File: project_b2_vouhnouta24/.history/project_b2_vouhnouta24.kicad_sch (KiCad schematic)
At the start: 7 parts, among them J1 AVR-ISP-10, U1 ATmega328-P-A, Y1 16Mhz

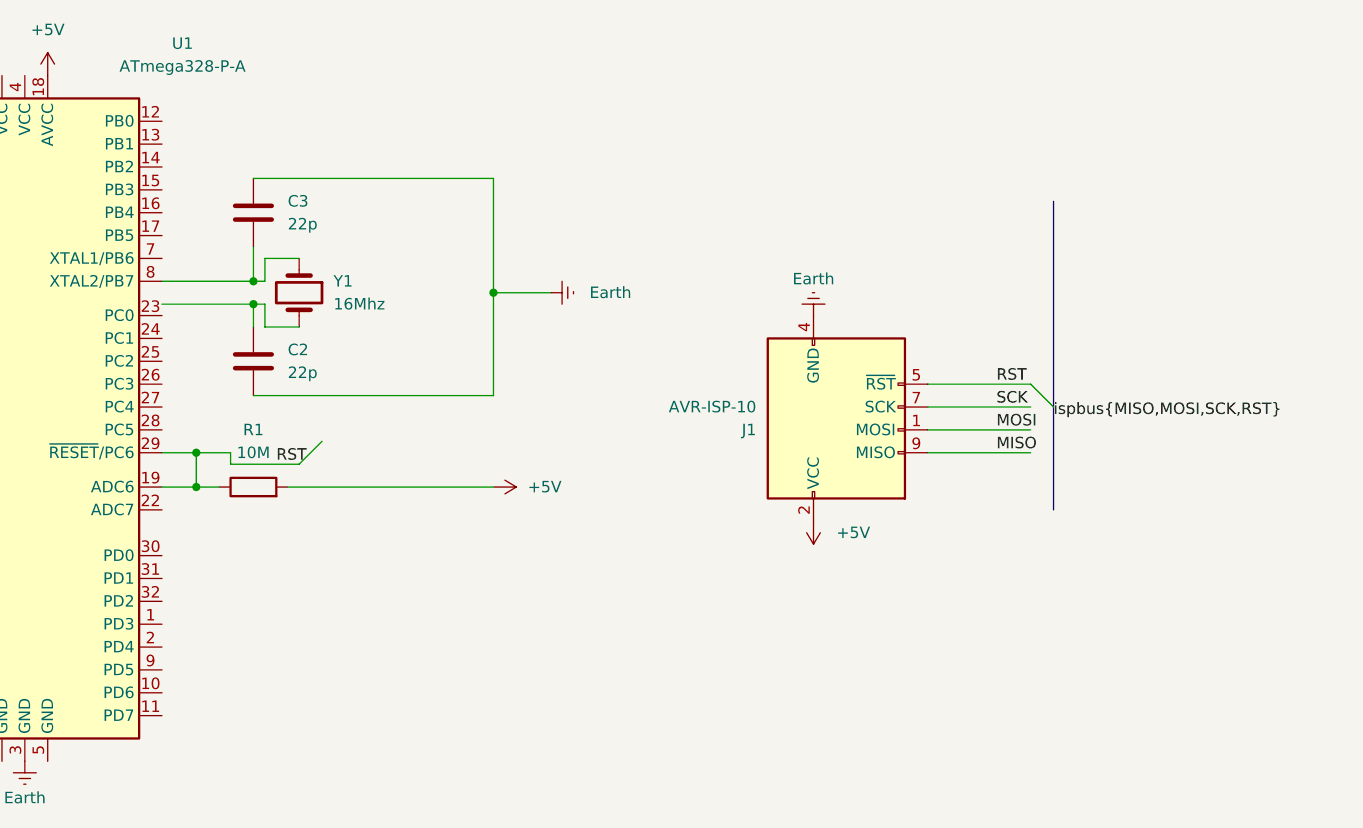
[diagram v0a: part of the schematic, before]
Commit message: J1 bus complete
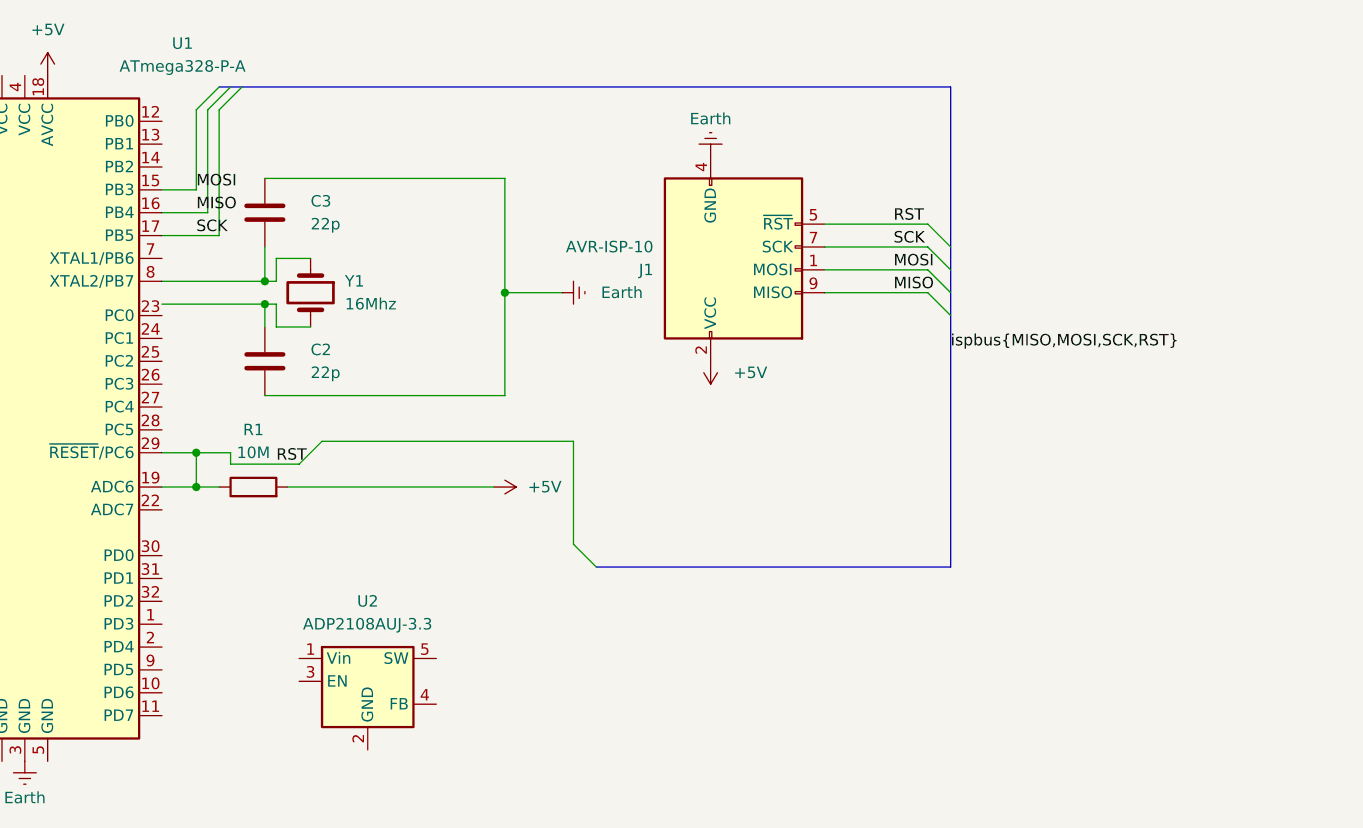
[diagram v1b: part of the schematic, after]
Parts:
- added U2: ADP2108AUJ-3.3, Package_TO_SOT_SMD:TSOT-23-5, symbol Regulator_Switching:ADP2108AUJ-3.3
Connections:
- net MISO: now also U1.16 (PB4)
- net MOSI: now also U1.15 (PB3)
- net SCK: now also U1.17 (PB5)
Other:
- moved on the sheet: C2, C3, J1, Y1

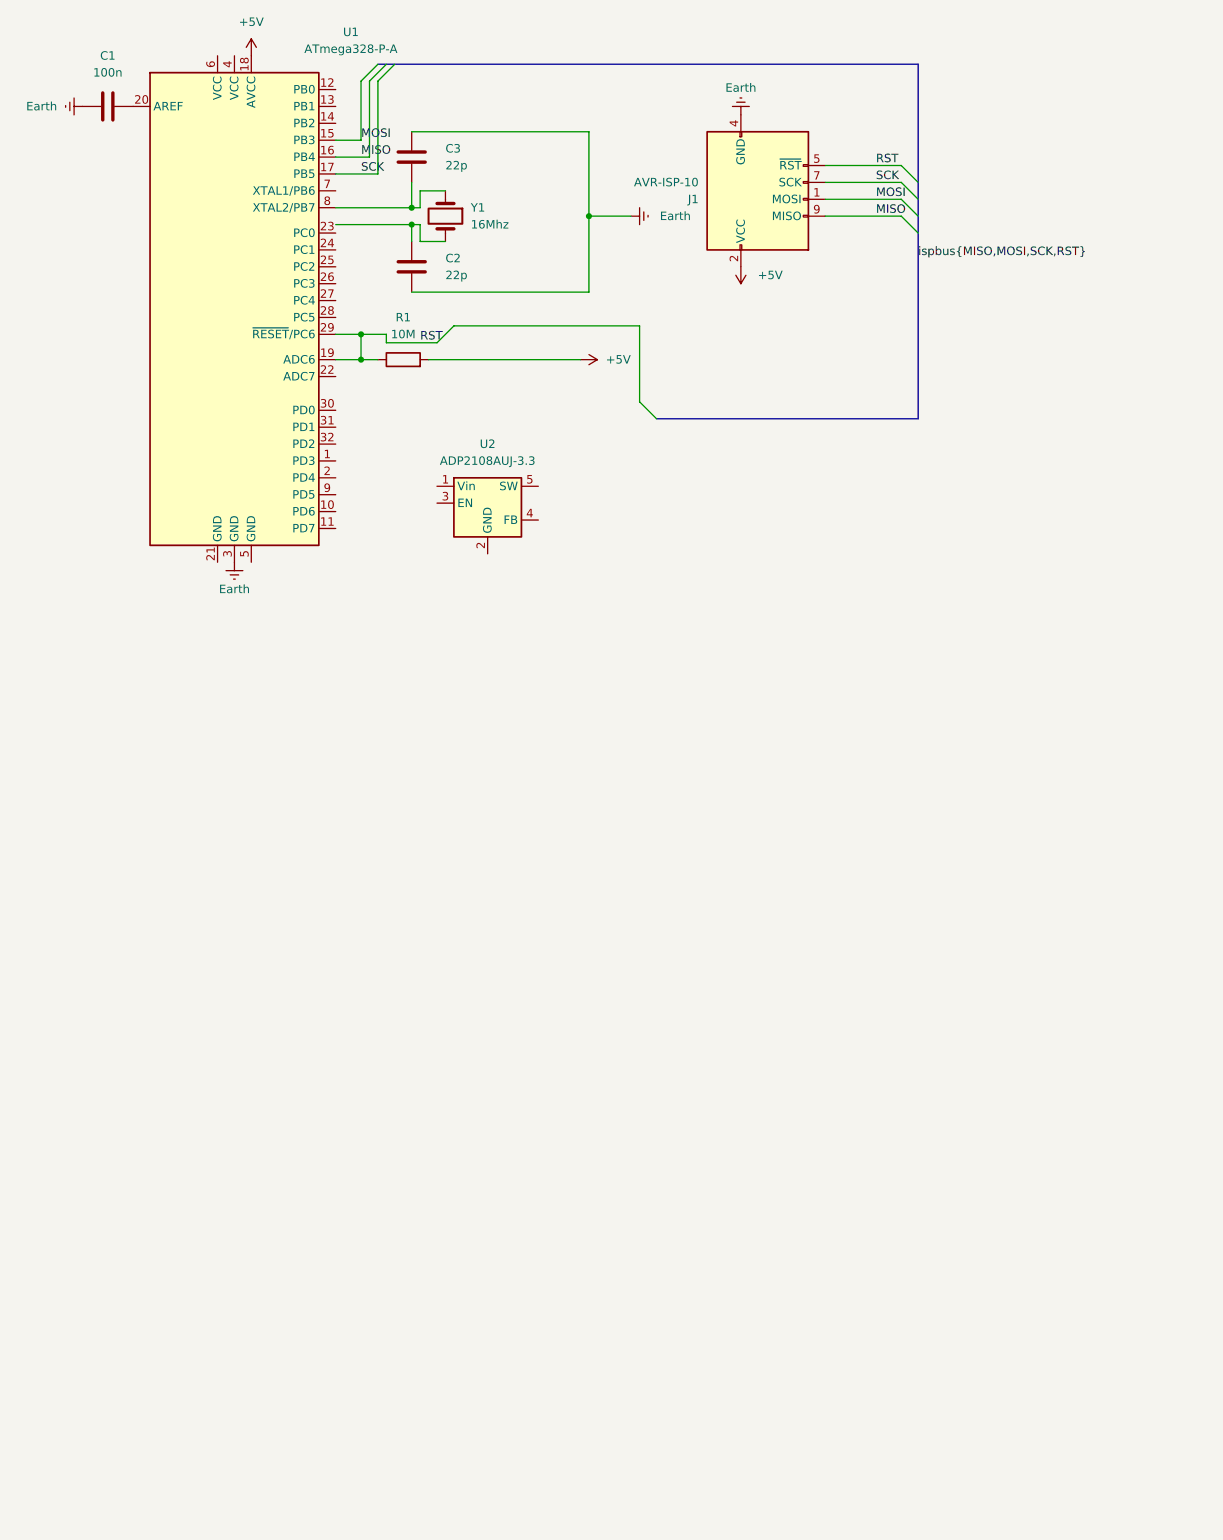
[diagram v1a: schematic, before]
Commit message: U2 modulator
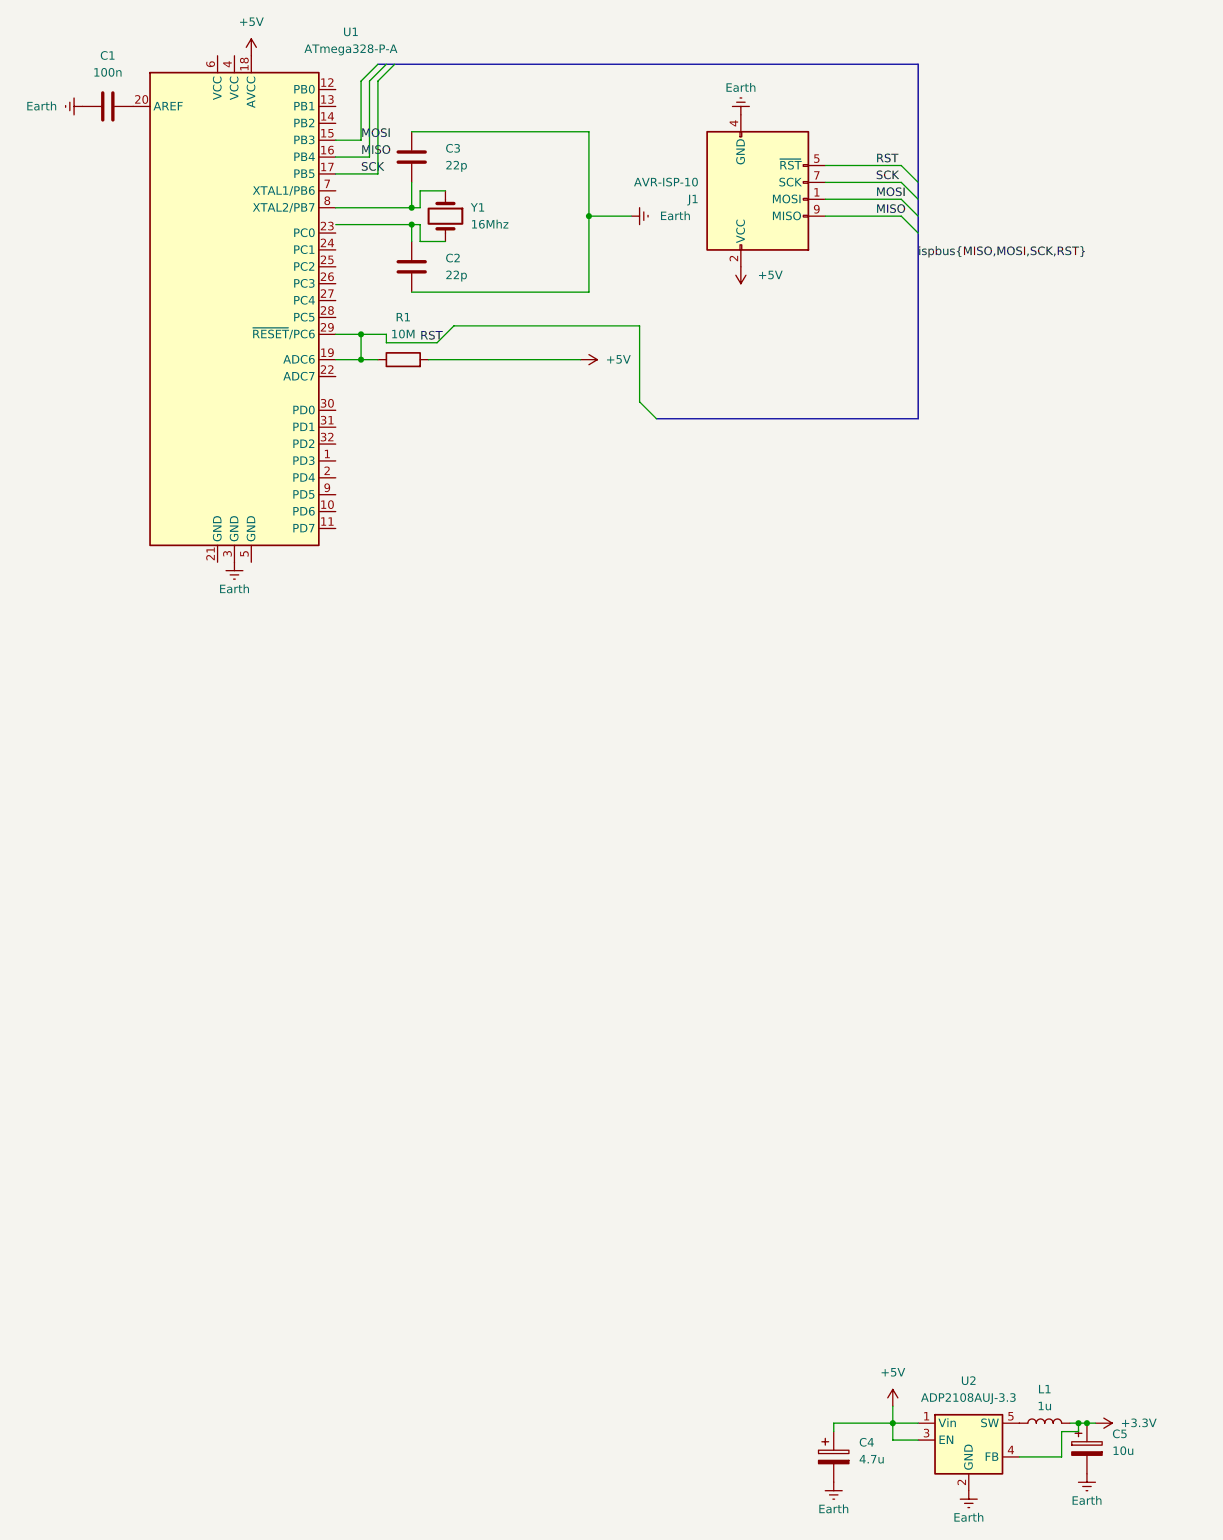
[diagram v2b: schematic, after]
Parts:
- added C4: 4.7u, Capacitor_THT:CP_Radial_D6.3mm_P2.50mm, symbol Device:C_Polarized
- added C5: 10u, Capacitor_THT:CP_Radial_D6.3mm_P2.50mm, symbol Device:C_Polarized
- added L1: 1u, Inductor_SMD:L_2010_5025Metric, symbol Device:L
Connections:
- net +5V: now also U2.1 (Vin), U2.3 (EN), C4.1
- net Earth: now also U2.2 (GND), C4.2, C5.2
- net +3.3V: now reaches U2.4 (FB)
- net +3.3V: now also C5.1, L1.2
- net at U2.5 (SW): now also L1.1
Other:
- moved on the sheet: U2
